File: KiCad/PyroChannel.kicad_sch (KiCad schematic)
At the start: 5 parts, among them Q1 IRLML0030

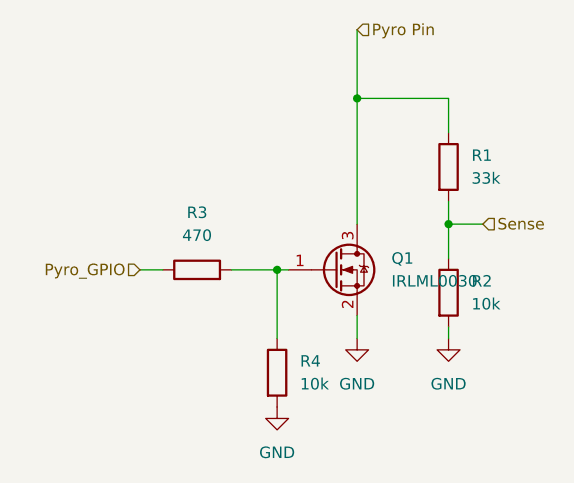
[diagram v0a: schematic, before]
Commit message: very rough sketch layout
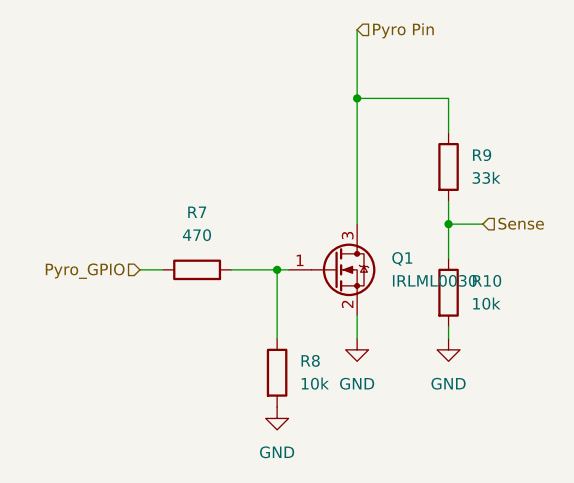
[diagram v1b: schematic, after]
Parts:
- renumbered R2 to R10, R3 to R7, R4 to R8, R1 to R9
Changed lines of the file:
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@@
 		(dnp no)
 		(fields_autoplaced yes)
-		(property "Reference" "#PWR03"
+		(property "Reference" "#PWR040"
 			(at 157.48 107.95 0)
 			(effects
@@
 			(project ""
 				(path "/16f8cce7-467e-4342-b55a-00af81cd6f69/fc7ffde7-f19b-4eb6-b923-3f87c2b4142b"
-					(reference "#PWR03")
+					(reference "#PWR040")
 					(unit 1)
 				)
@@
 		(dnp no)
 		(fields_autoplaced yes)
-		(property "Reference" "#PWR02"
+		(property "Reference" "#PWR039"
 			(at 147.32 107.95 0)
 			(effects
@@
 			(project ""
 				(path "/16f8cce7-467e-4342-b55a-00af81cd6f69/fc7ffde7-f19b-4eb6-b923-3f87c2b4142b"
-					(reference "#PWR02")
+					(reference "#PWR039")
 					(unit 1)
 				)
@@
 		(dnp no)
 		(fields_autoplaced yes)
-		(property "Reference" "R1"
+		(property "Reference" "R9"
 			(at 160.02 81.2799 0)
 			(effects
@@
 			(project ""
 				(path "/16f8cce7-467e-4342-b55a-00af81cd6f69/fc7ffde7-f19b-4eb6-b923-3f87c2b4142b"
-					(reference "R1")
+					(reference "R9")
 					(unit 1)
 				)
@@
 		(dnp no)
 		(fields_autoplaced yes)
-		(property "Reference" "#PWR01"
+		(property "Reference" "#PWR038"
 			(at 138.43 115.57 0)
 			(effects
@@
 			(project ""
 				(path "/16f8cce7-467e-4342-b55a-00af81cd6f69/fc7ffde7-f19b-4eb6-b923-3f87c2b4142b"
-					(reference "#PWR01")
+					(reference "#PWR038")
 					(unit 1)
 				)
@@
 		(dnp no)
 		(fields_autoplaced yes)
-		(property "Reference" "R3"
+		(property "Reference" "R7"
 			(at 129.54 87.63 90)
 			(effects
@@
 			(project ""
 				(path "/16f8cce7-467e-4342-b55a-00af81cd6f69/fc7ffde7-f19b-4eb6-b923-3f87c2b4142b"
-					(reference "R3")
+					(reference "R7")
 					(unit 1)
 				)
@@
 		(dnp no)
 		(fields_autoplaced yes)
-		(property "Reference" "R4"
+		(property "Reference" "R8"
 			(at 140.97 104.1399 0)
 			(effects
@@
 			(project ""
 				(path "/16f8cce7-467e-4342-b55a-00af81cd6f69/fc7ffde7-f19b-4eb6-b923-3f87c2b4142b"
-					(reference "R4")
+					(reference "R8")
 					(unit 1)
 				)
@@
 		(dnp no)
 		(fields_autoplaced yes)
-		(property "Reference" "R2"
+		(property "Reference" "R10"
 			(at 160.02 95.2499 0)
 			(effects
@@
 			(project ""
 				(path "/16f8cce7-467e-4342-b55a-00af81cd6f69/fc7ffde7-f19b-4eb6-b923-3f87c2b4142b"
-					(reference "R2")
-					(unit 1)
-				)
+					(reference "R10")
+					(unit 1)
+				)
